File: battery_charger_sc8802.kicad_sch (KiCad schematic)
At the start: 38 parts, among them Q1 Q_NMOS_GSD, Q2 Q_NMOS_GSD, Q3 Q_NMOS_GSD, Q4 Q_NMOS_GSD, U1 SC8802QDER

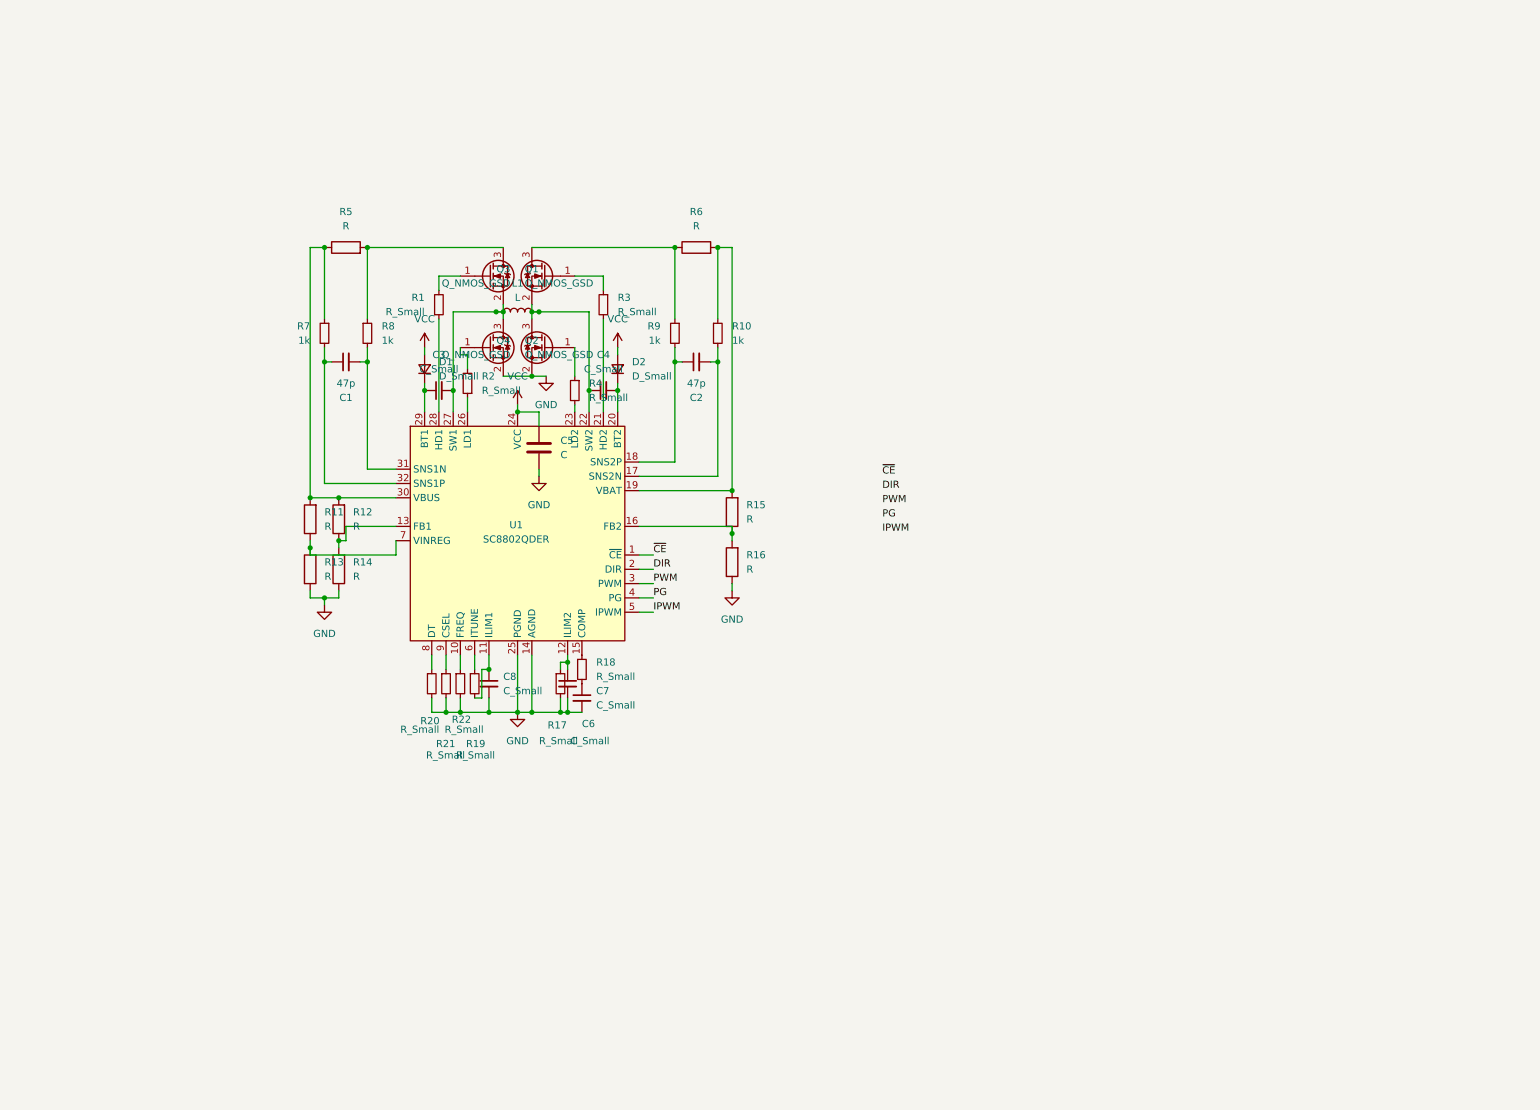
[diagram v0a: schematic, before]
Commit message: 添加电源，MCU和接口电路
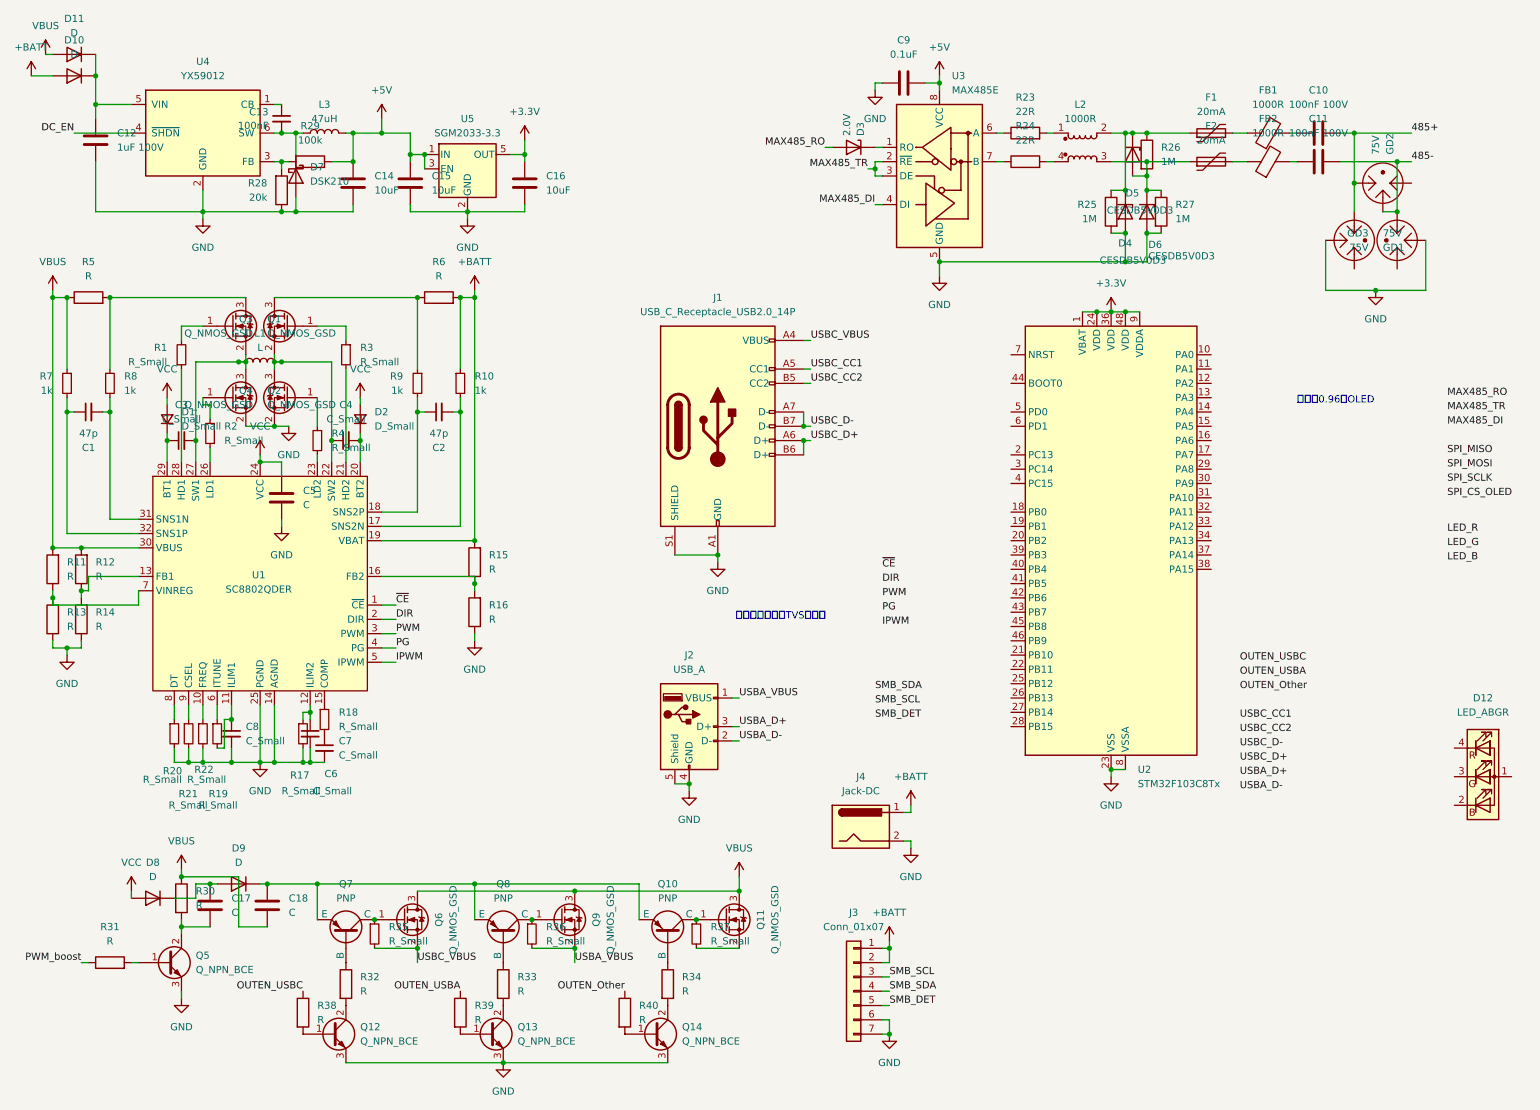
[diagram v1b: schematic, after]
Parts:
- added C10, C11: 100nF 100V, Capacitor_SMD:C_0603_1608Metric, symbol Device:C
- added C12: 1uF 100V, Capacitor_SMD:C_0805_2012Metric, symbol Device:C
- added C13: 100nF, Capacitor_SMD:C_0402_1005Metric, symbol Device:C_Small
- added C14, C15, C16: 10uF, Capacitor_SMD:C_0805_2012Metric, symbol Device:C
- added C17, C18: C, symbol Device:C
- added C9: 0.1uF, Capacitor_SMD:C_0603_1608Metric, symbol Device:C
- added D10, D11, D8, D9: D, symbol Device:D
- added D12: LED_ABGR, symbol Device:LED_ABGR
- added D3: 2.0V, Diode_SMD:D_SOD-323, symbol Device:D_Zener
- added D4, D5, D6: CESDB5V0D3, Diode_SMD:D_SOD-323, symbol Diode:ESD5Zxx
- added D7: DSK210, Diode_SMD:D_SOD-123F, symbol Device:D_Schottky
- added F1, F2: 20mA, Fuse:Fuse_0603_1608Metric, symbol Device:Polyfuse
- added FB1, FB2: 1000R, Inductor_SMD:L_0603_1608Metric, symbol Device:FerriteBead
- added GD1, GD2, GD3: 75V, Capacitor_SMD:C_1206_3216Metric, symbol Device:GDT_3Pin
- added J1: USB_C_Receptacle_USB2.0_14P, Connector_USB:USB_C_Receptacle_GCT_USB4115-03-C, symbol Connector:USB_C_Receptacle_USB2.0_14P
- added J2: USB_A, symbol Connector:USB_A
- added J3: Conn_01x07, symbol Connector_Generic:Conn_01x07
- added J4: Jack-DC, symbol Connector:Jack-DC
- added L2: 1000R, Inductor_SMD:L_CommonModeChoke_Coilcraft_1812CAN, symbol Device:L_Coupled_1243
- added L3: 47uH, Inductor_SMD:L_1210_3225Metric, symbol Device:L
- added Q10, Q7, Q8: PNP, symbol Simulation_SPICE:PNP
- added Q11, Q6, Q9: Q_NMOS_GSD, symbol Device:Q_NMOS_GSD
- added Q12, Q13, Q14, Q5: Q_NPN_BCE, symbol Device:Q_NPN_BCE
- added R23, R24: 22R, Resistor_SMD:R_0603_1608Metric, symbol Device:R
- added R25, R26, R27: 1M, Resistor_SMD:R_0603_1608Metric, symbol Device:R
- added R28: 20k, Resistor_SMD:R_0402_1005Metric, symbol Device:R
- added R29: 100k, Resistor_SMD:R_0402_1005Metric, symbol Device:R
- added R30, R31, R32, R33, R34, R38, R39, R40: R, symbol Device:R
- added R35, R36, R37: R_Small, symbol Device:R_Small
- added U2: STM32F103C8Tx, Package_QFP:LQFP-48_7x7mm_P0.5mm, symbol MCU_ST_STM32F1:STM32F103C8Tx
- added U3: MAX485E, Package_SO:SOIC-8_3.9x4.9mm_P1.27mm, symbol Interface_UART:MAX485E
- added U4: YX59012, Package_TO_SOT_SMD:SOT-23-6, symbol Regulator_Switching:LV2862XDDC
- added U5: SGM2033-3.3, Package_TO_SOT_SMD:SOT-23-5, symbol Regulator_Linear:TLV70033_SOT23-5
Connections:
- net GND: now also C12.1, C14.2, C15.2, C16.2, C9.1, D4.2 (A), D6.2 (A), D7.2 (A), GD1.2, GD3.2, J1.A1 (GND), J1.A12 (GND), J1.B1 (GND), J1.B12 (GND), J1.S1 (SHIELD), J2.4 (GND), J2.5 (Shield), J3.6 (Pin_6), J3.7 (Pin_7), J4.2, Q12.3 (E), Q13.3 (E), Q14.3 (E), Q5.3 (E), R25.2, R27.2, R28.1, U2.23 (VSS), U2.35 (VSS), U2.47 (VSS), U2.8 (VSSA), U3.5 (GND), U4.2 (GND), U5.2 (GND)
- net VCC: now also D8.2 (A)
- net +BATT: now reaches R10.1, R15.2, R6.2, U1.19 (VBAT)
- net +BATT: now also D10.2 (A), J3.1 (Pin_1), J3.2 (Pin_2), J4.1
- net VBUS: now reaches R11.2, R12.2, R5.1, R7.1, U1.30 (VBUS)
- net VBUS: now also C18.2, D11.2 (A), Q11.3 (D), Q6.3 (D), Q9.3 (D), R30.1
- new net: D3.1 (K), U3.1 (RO)
- new net: R23.1, U3.6 (A)
- new net: R24.1, U3.7 (B)
- new net: C17.2, Q5.2 (C), R30.2
- new net: C13.1, U4.1 (CB)
- new net: R28.2, R29.1, U4.3 (FB)
- new net: C12.2, D10.1 (K), D11.1 (K), U4.5 (VIN)
- new net: C13.2, D7.1 (K), L3.1, U4.6 (SW)
- new net: D4.1 (K), D5.1 (K), F1.1, L2.2, R25.1, R26.1
- new net: Q14.1 (B), R40.2
- new net: Q14.2 (C), R34.2
- new net: Q13.1 (B), R39.2
- new net: Q13.2 (C), R33.2
- new net: Q5.1 (B), R31.2
- new net: Q12.1 (B), R38.2
- new net: Q12.2 (C), R32.2
- new net: Q10.1 (C), Q11.1 (G), R37.1
- new net: Q11.2 (S), R37.2
- new net: Q7.2 (B), R32.1
- new net: C11.1, FB2.2
- new net: D5.2 (A), D6.1 (K), F2.1, L2.3, R26.2, R27.1
- new net: C10.1, FB1.2
- new net: L2.1, R23.2
- new net: Q8.2 (B), R33.1
- new net: F1.2, FB1.1
- new net: Q10.2 (B), R34.1
- new net: C18.1, D9.1 (K), Q10.3 (E), Q7.3 (E), Q8.3 (E)
- new net: C17.1, D8.1 (K), D9.2 (A)
- new net: Q6.1 (G), Q7.1 (C), R35.1
- new net: L2.4, R24.2
- new net: Q8.1 (C), Q9.1 (G), R36.1
- new net: F2.2, FB2.1
- new net +3.3V: C16.1, U2.1 (VBAT), U2.24 (VDD), U2.36 (VDD), U2.48 (VDD), U2.9 (VDDA), U5.5 (OUT)
- new net +5V: C14.1, C15.1, C9.2, L3.2, R29.2, U3.8 (VCC), U5.1 (IN), U5.3 (EN)
- new net 485+: C10.2, GD1.1, GD2.1
- new net 485-: C11.2, GD2.2, GD3.1
- new net DC_EN: U4.4 (~{SHDN})
- new net MAX485_DI: U3.4 (DI)
- new net MAX485_RO: D3.2 (A)
- new net MAX485_TR: U3.2 (~{RE}), U3.3 (DE)
- new net OUTEN_Other: R40.1
- new net OUTEN_USBA: R39.1
- new net OUTEN_USBC: R38.1
- new net PWM_boost: R31.1
- new net SMB_DET: J3.5 (Pin_5)
- new net SMB_SCL: J3.3 (Pin_3)
- new net SMB_SDA: J3.4 (Pin_4)
- new net USBA_D+: J2.3 (D+)
- new net USBA_D-: J2.2 (D-)
- new net USBA_VBUS: J2.1 (VBUS), Q9.2 (S), R36.2
- new net USBC_CC1: J1.A5 (CC1)
- new net USBC_CC2: J1.B5 (CC2)
- new net USBC_D+: J1.A6 (D+), J1.B6 (D+)
- new net USBC_D-: J1.A7 (D-), J1.B7 (D-)
- new net USBC_VBUS: J1.A4 (VBUS), J1.A9 (VBUS), J1.B4 (VBUS), J1.B9 (VBUS), Q6.2 (S), R35.2
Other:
- note added: "待添加0.96寸OLED"
- note added: "接口电路待添加TVS等保护"
- moved on the sheet: C1, C2, C3, C4, C5, C6, C7, C8, D1, D2, L1, Q1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

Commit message: 分配元器件封装
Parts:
- C1, C2, C3, C4, C6, C7, C8: footprint (none) -> Capacitor_SMD:C_0402_1005Metric
- C17, C18, C5: footprint (none) -> Capacitor_SMD:C_0603_1608Metric
- D1, D2: footprint (none) -> Diode_SMD:D_SOD-523
- D10, D11, D8, D9: footprint (none) -> Diode_SMD:D_SOD-323
- D12: footprint (none) -> LED_SMD:LED_RGB_1210
- J2: footprint (none) -> Connector_USB:USB_A_Molex_67643_Horizontal
- J3: footprint (none) -> Connector_PinHeader_2.54mm:PinHeader_1x07_P2.54mm_Vertical
- J4: footprint (none) -> Connector_BarrelJack:BarrelJack_GCT_DCJ200-10-A_Horizontal
- L1: footprint (none) -> Inductor_SMD:L_APV_ANR8065
- Q1, Q2, Q3, Q4: footprint (none) -> Package_TO_SOT_SMD:TO-252-2
- Q10, Q11, Q12, Q13, Q14, Q5, Q6, Q7, Q8, Q9: footprint (none) -> Package_TO_SOT_SMD:SOT-23
- R1, R10, R17, R18, R19, R2, R20, R21, R22, R3, R31, R35, R36, R37, R38, R39, R4, R40, R7, R8, R9: footprint (none) -> Resistor_SMD:R_0402_1005Metric
- R11, R12, R13, R14, R15, R16, R30, R32, R33, R34: footprint (none) -> Resistor_SMD:R_0603_1608Metric
- R5, R6: footprint (none) -> Resistor_SMD:R_1206_3216Metric
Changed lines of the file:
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@@
 			)
 		)
-		(property "Footprint" ""
+		(property "Footprint" "Resistor_SMD:R_0603_1608Metric"
 			(at 94.488 106.68 90)
 			(effects
@@
 			)
 		)
-		(property "Footprint" ""
+		(property "Footprint" "Resistor_SMD:R_0603_1608Metric"
 			(at 19.558 116.84 90)
 			(effects
@@
 			)
 		)
-		(property "Footprint" ""
+		(property "Footprint" "Resistor_SMD:R_0603_1608Metric"
 			(at 38.862 166.37 90)
 			(effects
@@
 			)
 		)
-		(property "Footprint" ""
+		(property "Footprint" "Package_TO_SOT_SMD:TO-252-2"
 			(at 54.61 62.23 0)
 			(effects
@@
 			)
 		)
-		(property "Footprint" ""
+		(property "Footprint" "Diode_SMD:D_SOD-523"
 			(at 38.1 81.28 90)
 			(effects
@@
 			)
 		)
-		(property "Footprint" ""
+		(property "Footprint" "Capacitor_SMD:C_0402_1005Metric"
 			(at 40.64 85.09 0)
 			(effects
@@
 			)
 		)
-		(property "Footprint" ""
+		(property "Footprint" "Resistor_SMD:R_0402_1005Metric"
 			(at 90.17 74.93 0)
 			(effects
@@
 			)
 		)
-		(property "Footprint" ""
+		(property "Footprint" "Resistor_SMD:R_0603_1608Metric"
 			(at 94.488 115.57 90)
 			(effects
@@
 			)
 		)
-		(property "Footprint" ""
+		(property "Footprint" "Package_TO_SOT_SMD:SOT-23"
 			(at 129.54 187.96 0)
 			(effects
@@
 			)
 		)
-		(property "Footprint" ""
+		(property "Footprint" "Package_TO_SOT_SMD:SOT-23"
 			(at 100.33 187.96 0)
 			(effects
@@
 			)
 		)
-		(property "Footprint" ""
+		(property "Footprint" "Resistor_SMD:R_0402_1005Metric"
 			(at 27.94 179.578 90)
 			(effects
@@
 			)
 		)
-		(property "Footprint" ""
+		(property "Footprint" "Package_TO_SOT_SMD:SOT-23"
 			(at 72.39 187.96 0)
 			(effects
@@
 			)
 		)
-		(property "Footprint" ""
+		(property "Footprint" "Resistor_SMD:R_0402_1005Metric"
 			(at 132.08 172.72 0)
 			(effects
@@
 			)
 		)
-		(property "Footprint" ""
+		(property "Footprint" "Resistor_SMD:R_0603_1608Metric"
 			(at 24.638 107.95 90)
 			(effects
@@
 			)
 		)
-		(property "Footprint" ""
+		(property "Footprint" "Resistor_SMD:R_0603_1608Metric"
 			(at 68.072 181.61 90)
 			(effects
@@
 			)
 		)
-		(property "Footprint" ""
+		(property "Footprint" "Resistor_SMD:R_0402_1005Metric"
 			(at 40.64 69.85 0)
 			(effects
@@
 			)
 		)
-		(property "Footprint" ""
+		(property "Footprint" "Resistor_SMD:R_0402_1005Metric"
 			(at 45.72 83.82 0)
 			(effects
@@
 			)
 		)
-		(property "Footprint" ""
+		(property "Footprint" "LED_SMD:LED_RGB_1210"
 			(at 271.78 146.05 0)
 			(effects
@@
 			)
 		)
-		(property "Footprint" ""
+		(property "Footprint" "Resistor_SMD:R_0402_1005Metric"
 			(at 20.32 74.93 0)
 			(effects
@@
 			)
 		)
-		(property "Footprint" ""
+		(property "Footprint" "Resistor_SMD:R_0603_1608Metric"
 			(at 96.012 181.61 90)
 			(effects
@@
 			)
 		)
-		(property "Footprint" ""
+		(property "Footprint" "Inductor_SMD:L_APV_ANR8065"
 			(at 54.61 71.12 0)
 			(effects
@@
 			)
 		)
-		(property "Footprint" ""
+		(property "Footprint" "Connector_PinHeader_2.54mm:PinHeader_1x07_P2.54mm_Vertical"
 			(at 160.02 182.88 0)
 			(effects
@@
 			)
 		)
-		(property "Footprint" ""
+		(property "Footprint" "Resistor_SMD:R_0402_1005Metric"
 			(at 88.392 186.69 90)
 			(effects
@@
 			)
 		)
-		(property "Footprint" ""
+		(property "Footprint" "Package_TO_SOT_SMD:SOT-23"
 			(at 127 137.16 0)
 			(effects
@@
 			)
 		)
-		(property "Footprint" ""
+		(property "Footprint" "Capacitor_SMD:C_0603_1608Metric"
 			(at 46.6852 171.45 0)
 			(effects
@@
 			)
 		)
-		(property "Footprint" ""
+		(property "Footprint" "Resistor_SMD:R_0402_1005Metric"
 			(at 39.37 137.16 0)
 			(effects
@@
 			)
 		)
-		(property "Footprint" ""
+		(property "Footprint" "Package_TO_SOT_SMD:SOT-23"
 			(at 85.09 167.64 0)
 			(effects
@@
 			)
 		)
-		(property "Footprint" ""
+		(property "Footprint" "Resistor_SMD:R_0603_1608Metric"
 			(at 19.558 107.95 90)
 			(effects
@@
 			)
 		)
-		(property "Footprint" ""
+		(property "Footprint" "Capacitor_SMD:C_0402_1005Metric"
 			(at 86.36 80.01 0)
 			(effects
@@
 			)
 		)
-		(property "Footprint" ""
+		(property "Footprint" "Capacitor_SMD:C_0603_1608Metric"
 			(at 57.4548 91.44 0)
 			(effects
@@
 			)
 		)
-		(property "Footprint" ""
+		(property "Footprint" "Diode_SMD:D_SOD-523"
 			(at 72.39 81.28 90)
 			(effects
@@
 			)
 		)
-		(property "Footprint" ""
+		(property "Footprint" "Resistor_SMD:R_0402_1005Metric"
 			(at 41.91 137.16 0)
 			(effects
@@
 			)
 		)
-		(property "Footprint" ""
+		(property "Footprint" "Capacitor_SMD:C_0603_1608Metric"
 			(at 56.8452 171.45 0)
 			(effects
@@
 			)
 		)
-		(property "Footprint" ""
+		(property "Footprint" "Resistor_SMD:R_0603_1608Metric"
 			(at 125.222 181.61 90)
 			(effects
@@
 			)
 		)
-		(property "Footprint" ""
+		(property "Footprint" "Package_TO_SOT_SMD:TO-252-2"
 			(at 54.61 62.23 0)
 			(effects
@@
 			)
 		)
-		(property "Footprint" ""
+		(property "Footprint" "Resistor_SMD:R_0402_1005Metric"
 			(at 74.93 172.72 0)
 			(effects
@@
 			)
 		)
-		(property "Footprint" ""
+		(property "Footprint" "Resistor_SMD:R_0402_1005Metric"
 			(at 46.99 137.16 0)
 			(effects
@@
 			)
 		)
-		(property "Footprint" ""
+		(property "Footprint" "Resistor_SMD:R_0603_1608Metric"
 			(at 24.638 116.84 90)
 			(effects
@@
 			)
 		)
-		(property "Footprint" ""
+		(property "Footprint" "Resistor_SMD:R_0402_1005Metric"
 			(at 102.87 172.72 0)
 			(effects
@@
 			)
 		)
-		(property "Footprint" ""
+		(property "Footprint" "Resistor_SMD:R_0402_1005Metric"
 			(at 66.04 134.62 0)
 			(effects
@@
 			)
 		)
-		(property "Footprint" ""
+		(property "Footprint" "Package_TO_SOT_SMD:TO-252-2"
 			(at 54.61 74.93 0)
 			(effects
@@
 			)
 		)
-		(property "Footprint" ""
+		(property "Footprint" "Resistor_SMD:R_1206_3216Metric"
 			(at 86.36 61.468 90)
 			(effects
@@
 			)
 		)
-		(property "Footprint" ""
+		(property "Footprint" "Capacitor_SMD:C_0402_1005Metric"
 			(at 63.5 137.16 0)
 			(effects
@@
 			)
 		)
-		(property "Footprint" ""
+		(property "Footprint" "Resistor_SMD:R_0402_1005Metric"
 			(at 117.602 186.69 90)
 			(effects
@@
 			)
 		)
-		(property "Footprint" ""
+		(property "Footprint" "Capacitor_SMD:C_0402_1005Metric"
 			(at 49.53 137.16 0)
 			(effects
@@
 			)
 		)
-		(property "Footprint" ""
+		(property "Footprint" "Resistor_SMD:R_0402_1005Metric"
 			(at 60.452 186.69 90)
 			(effects
@@
 			)
 		)
-		(property "Footprint" ""
+		(property "Footprint" "Package_TO_SOT_SMD:SOT-23"
 			(at 142.24 167.64 0)
 			(effects
@@
 			)
 		)
-		(property "Footprint" ""
+		(property "Footprint" "Resistor_SMD:R_1206_3216Metric"
 			(at 24.13 61.468 90)
 			(effects
@@
 			)
 		)
-		(property "Footprint" ""
+		(property "Footprint" "Resistor_SMD:R_0402_1005Metric"
 			(at 27.94 74.93 0)
 			(effects
@@
 			)
 		)
-		(property "Footprint" ""
+		(property "Footprint" "Package_TO_SOT_SMD:SOT-23"
 			(at 97.79 137.16 0)
 			(effects
@@
 			)
 		)
-		(property "Footprint" ""
+		(property "Footprint" "Package_TO_SOT_SMD:TO-252-2"
 			(at 54.61 74.93 0)
 			(effects
@@
 			)
 		)
-		(property "Footprint" ""
+		(property "Footprint" "Resistor_SMD:R_0402_1005Metric"
 			(at 62.23 137.16 0)
 			(effects
@@
 			)
 		)
-		(property "Footprint" ""
+		(property "Footprint" "Capacitor_SMD:C_0402_1005Metric"
 			(at 24.13 80.01 0)
 			(effects
@@
 			)
 		)
-		(property "Footprint" ""
+		(property "Footprint" "Diode_SMD:D_SOD-323"
 			(at 35.56 166.37 0)
 			(effects
@@
 			)
 		)
-		(property "Footprint" ""
+		(property "Footprint" "Package_TO_SOT_SMD:SOT-23"
 			(at 113.03 167.64 0)
 			(effects
@@
 			)
 		)
-		(property "Footprint" ""
+		(property "Footprint" "Resistor_SMD:R_0402_1005Metric"
 			(at 64.77 85.09 0)
 			(effects
@@
 			)
 		)
-		(property "Footprint" ""
+		(property "Footprint" "Capacitor_SMD:C_0402_1005Metric"
 			(at 69.85 85.09 0)
 			(effects
@@
 			)
 		)
-		(property "Footprint" ""
+		(property "Footprint" "Capacitor_SMD:C_0402_1005Metric"
 			(at 66.04 139.7 0)
 			(effects
@@
 			)
 		)
-		(property "Footprint" ""
+		(property "Footprint" "Connector_USB:USB_A_Molex_67643_Horizontal"
 			(at 134.62 137.16 0)
 			(effects
@@
 			)
 		)
-		(property "Footprint" ""
+		(property "Footprint" "Diode_SMD:D_SOD-323"
 			(at 50.8 163.83 0)
 			(effects
@@
 			)
 		)
-		(property "Footprint" ""
+		(property "Footprint" "Resistor_SMD:R_0402_1005Metric"
 			(at 44.45 137.16 0)
 			(effects
@@
 			)
 		)
-		(property "Footprint" ""
+		(property "Footprint" "Diode_SMD:D_SOD-323"
 			(at 21.59 20.32 0)
 			(effects
@@
 			)
 		)
-		(property "Footprint" ""
+		(property "Footprint" "Resistor_SMD:R_0402_1005Metric"
 			(at 69.85 69.85 0)
 			(effects
@@
 			)
 		)
-		(property "Footprint" ""
+		(property "Footprint" "Diode_SMD:D_SOD-323"
 			(at 21.59 16.51 0)
 			(effects
@@
 			)
 		)
-		(property "Footprint" ""
+		(property "Footprint" "Package_TO_SOT_SMD:SOT-23"
 			(at 43.18 175.26 0)
 			(effects
@@
 			)
 		)
-		(property "Footprint" ""
+		(property "Footprint" "Connector_BarrelJack:BarrelJack_GCT_DCJ200-10-A_Horizontal"
 			(at 162.56 154.686 0)
 			(effects
@@
 			)
 		)
-		(property "Footprint" ""
+		(property "Footprint" "Resistor_SMD:R_0402_1005Metric"
 			(at 82.55 74.93 0)
 			(effects
@@
 			)
 		)
-		(property "Footprint" ""
+		(property "Footprint" "Package_TO_SOT_SMD:SOT-23"
 			(at 69.85 137.16 0)
 			(effects

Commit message: PCB元器件分组和局部布局
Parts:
- J1: footprint Connector_USB:USB_C_Receptacle_GCT_USB4115-03-C -> Connector_USB:USB_C_Receptacle_HRO_TYPE-C-31-M-12
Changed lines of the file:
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@@
 			)
 		)
-		(property "Footprint" "Connector_USB:USB_C_Receptacle_GCT_USB4115-03-C"
+		(property "Footprint" "Connector_USB:USB_C_Receptacle_HRO_TYPE-C-31-M-12"
 			(at 139.7 82.55 0)
 			(effects
